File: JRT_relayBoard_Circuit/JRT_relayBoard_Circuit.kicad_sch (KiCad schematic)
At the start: 8 parts, among them J1 Conn_ESP32_Left, J2 Conn_ESP32_Right, J3 eCON_D1-4, J4 eCON_D5-8, J5 eCON_D9-12, J6 eCON_D13-15, J7 eCON_A1-4, J8 eCON_A5_UART_Vin_Vout

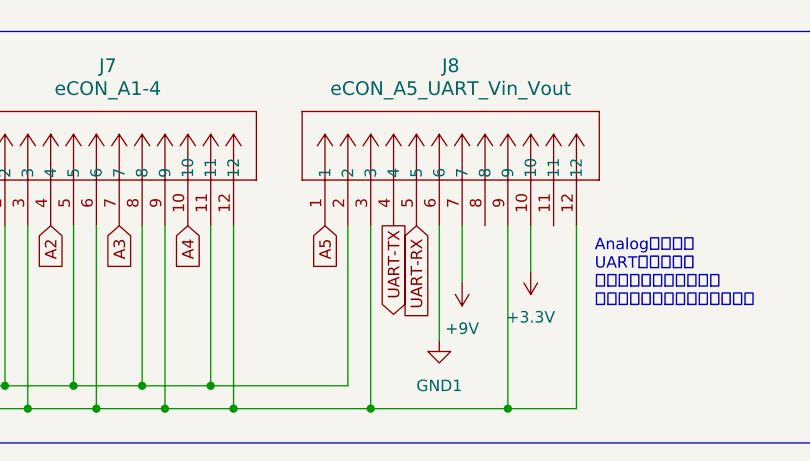
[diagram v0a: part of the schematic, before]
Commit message: 配線を行った
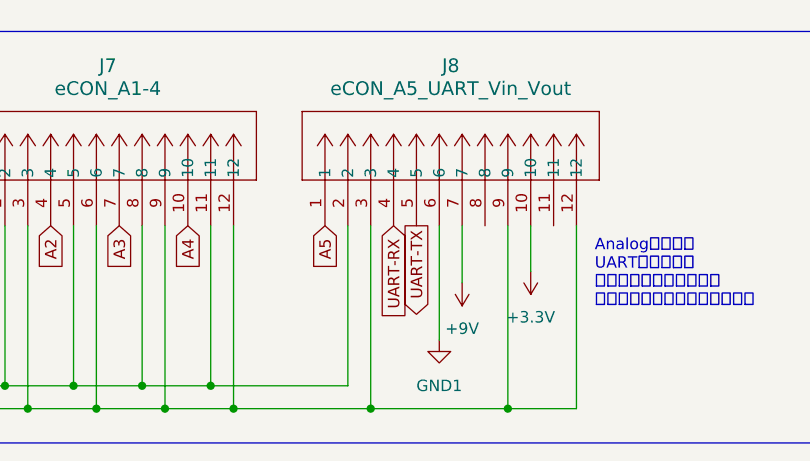
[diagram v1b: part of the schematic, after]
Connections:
- net UART-RX: now also J8.4; no longer J8.5
- net UART-TX: now also J8.5; no longer J8.4
